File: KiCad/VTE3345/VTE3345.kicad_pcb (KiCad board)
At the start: 2 copper layers, 58.4 x 55.9 mm, 26 parts, among them J1 Program, J2 Keypad, J3 Display, J4 Power, Q1 IRF540N, Q2 BD138, SW1 Reset, SW2 Mode, SW3 Switch, U1 ESP-12F, U2 AMS1117-3.3

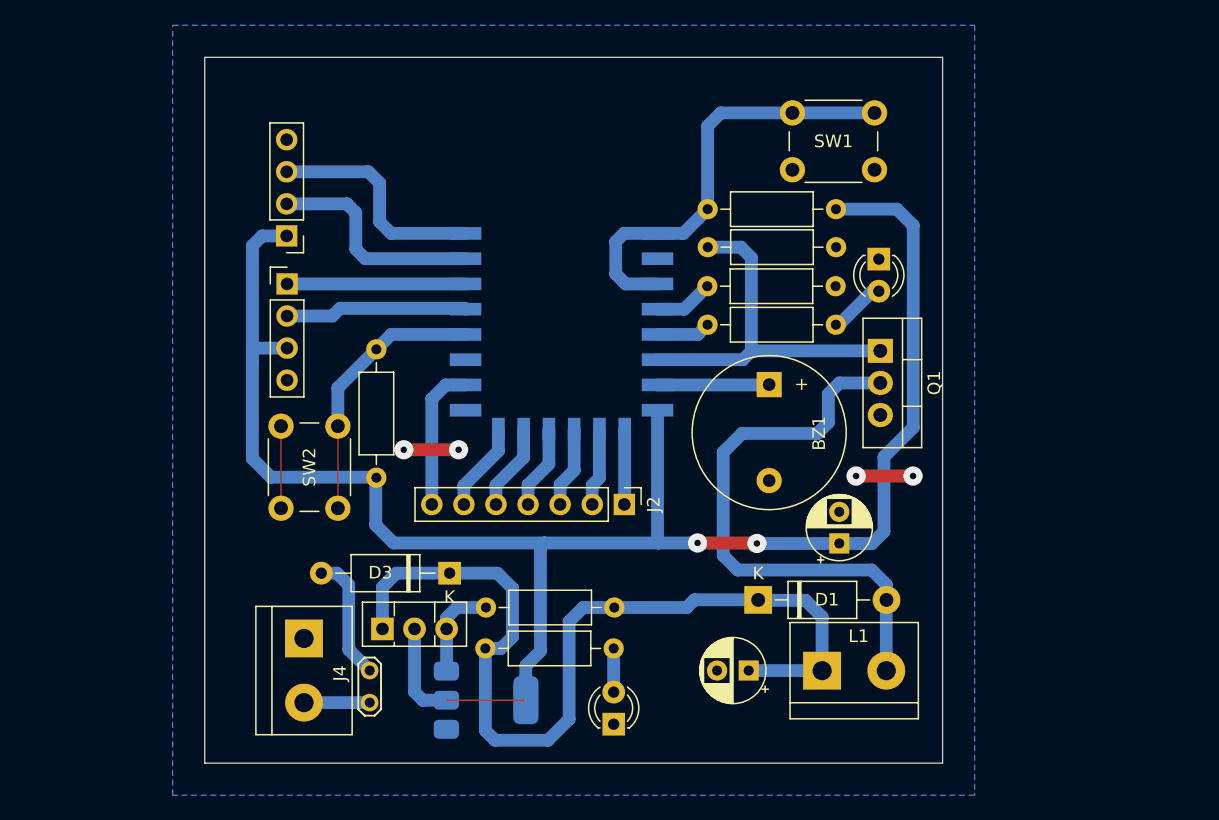
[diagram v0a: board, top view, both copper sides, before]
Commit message: Updates
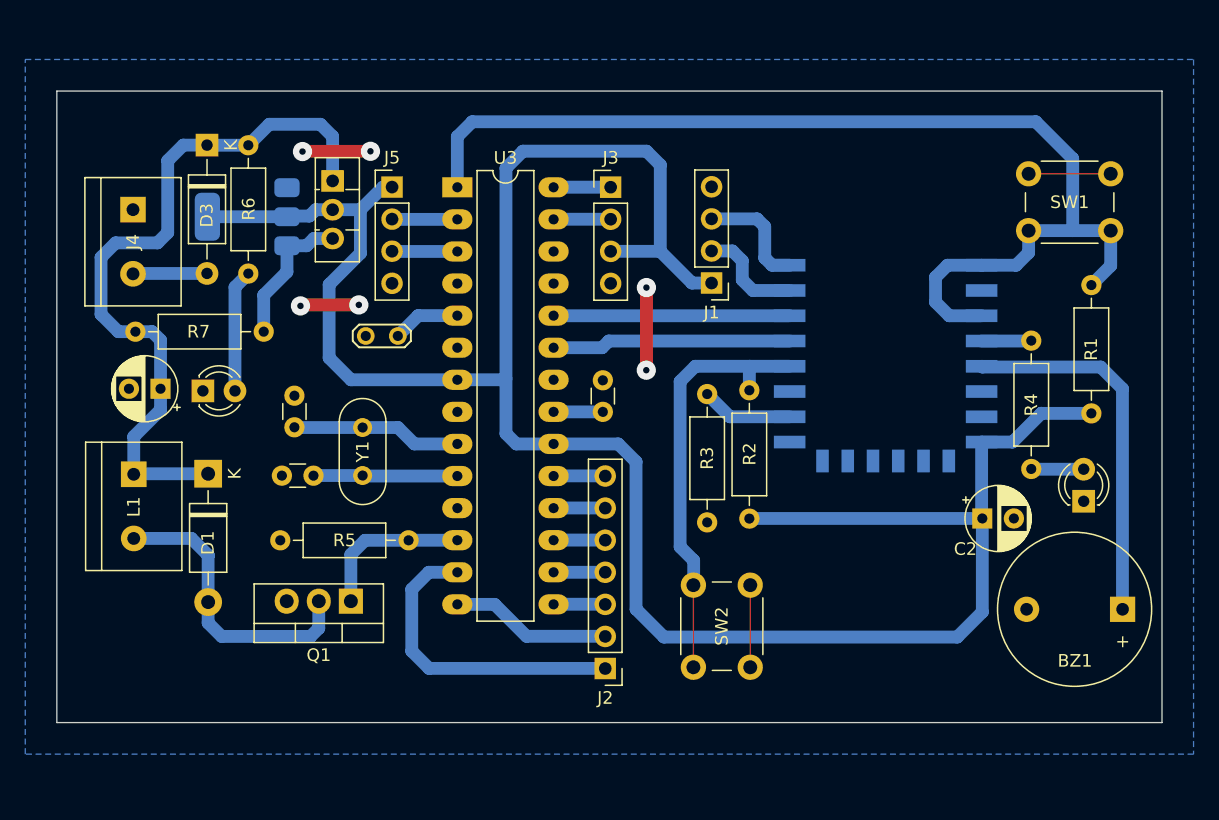
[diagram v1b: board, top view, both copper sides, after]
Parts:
- removed SW3: Switch, TestPoint:TestPoint_2Pads_Pitch2.54mm_Drill0.8mm
- added C3: 22pF, Capacitor_THT:C_Disc_D3.0mm_W1.6mm_P2.50mm, F.Cu at (126.7, 96.9)
- added C4: 22pF, Capacitor_THT:C_Disc_D3.0mm_W1.6mm_P2.50mm, F.Cu at (128.2, 100.7)
- added C5: 100nF, Capacitor_THT:C_Disc_D3.0mm_W1.6mm_P2.50mm, F.Cu at (151.2, 95.7)
- added J5: Program, Connector_PinHeader_2.54mm:PinHeader_1x04_P2.54mm_Vertical, F.Cu at (134.5, 77.9)
- added SW4: BTN, TestPoint:TestPoint_2Pads_Pitch2.54mm_Drill0.8mm, F.Cu at (134.9, 89.7)
- added U3: ATmega328P-P, Package_DIP:DIP-28_W7.62mm_LongPads, F.Cu at (139.6, 77.9)
- added Y1: 16MHz, Crystal:Crystal_HC52-U_Vertical, F.Cu at (132.1, 100.7)
- J1: value Program -> Program ESP
- moved L1 56.7 mm to (114.0, 100.6), turned to -90 degrees
- moved C1 51.6 mm to (116.1, 93.8)
- moved R5 49.8 mm to (125.6, 105.8), turned to 0 degrees
- moved Q1 46.4 mm to (131.2, 110.7), turned to 180 degrees
- moved D1 44.7 mm to (119.9, 100.6), turned to -90 degrees
- moved R6 44.0 mm to (123.1, 74.5), turned to -90 degrees
- moved R7 43.8 mm to (114.2, 89.3), turned to 0 degrees
- moved U2 42.7 mm to (123.0, 80.2), turned to 180 degrees
- moved D4 41.9 mm to (119.5, 94.0), turned to 0 degrees
- moved D3 39.0 mm to (119.8, 74.5), turned to -90 degrees
- moved J4 36.6 mm to (114.0, 79.7)
- moved Q2 35.7 mm to (129.8, 77.4), turned to -90 degrees
- moved SW2 34.0 mm to (158.3, 115.9), turned to 90 degrees
- moved J1 33.8 mm to (159.8, 85.5)
- moved BZ1 33.2 mm to (192.3, 111.3), turned to 180 degrees
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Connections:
- net /Rx renamed /RXD
- net /Tx renamed /TXD
- net Net-(SW1-B) renamed /reset
- J2 pad 1: /row1 -> /keypad_pin
- J2 pad 2: /row2 -> Net-(J2-Pin_2)
- J2 pad 3: /row3 -> Net-(J2-Pin_3)
- J2 pad 4: /row4 -> Net-(J2-Pin_4)
- J2 pad 5: /col1 -> Net-(J2-Pin_5)
- J2 pad 6: /col2 -> Net-(J2-Pin_6)
- J2 pad 7: /col3 -> Net-(J2-Pin_7)
- J4 pad 2: Net-(J4-Pin_2) -> Net-(D3-A)
- R3 pad 1: Net-(U1-GPIO16) -> Net-(U1-GPIO15)
- R4 pad 1: Net-(U1-GPIO14) -> Net-(U1-GPIO16)
- U1 pad 10: /row2 -> unconnected-(U1-MISO-Pad10)
- U1 pad 11: /row3 -> unconnected-(U1-GPIO9-Pad11)
- U1 pad 12: /row4 -> unconnected-(U1-GPIO10-Pad12)
- U1 pad 13: /col1 -> unconnected-(U1-MOSI-Pad13)
- U1 pad 14: /col2 -> unconnected-(U1-SCLK-Pad14)
- U1 pad 16: /col3 -> Net-(U1-GPIO15)
- U1 pad 19: /SDA -> /RxD
- U1 pad 20: /SCL -> /TxD
- U1 pad 5: Net-(U1-GPIO14) -> Net-(BZ1-+)
- U1 pad 6: Net-(Q1-G) -> unconnected-(U1-GPIO12-Pad6)
- U1 pad 7: Net-(BZ1-+) -> unconnected-(U1-GPIO13-Pad7)
- U1 pad 9: /row1 -> unconnected-(U1-CS0-Pad9)
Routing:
- net /reset: track 34.8 -> 87.6 mm
- net +3.3V: track 149.0 -> 187.2 mm, vias 4 -> 0
- net /keypad_pin: track 0.00 -> 25.0 mm
- net Net-(D1-A): track 44.9 -> 23.4 mm
- net Net-(BZ1-+): track 8.85 -> 29.4 mm
- net /RxD: track 0.00 -> 18.9 mm
- net /TxD: track 0.00 -> 18.7 mm
- net +12V: track 74.2 -> 57.5 mm
- net Net-(Q1-G): track 29.1 -> 12.6 mm
- net GND: track 15.3 -> 29.6 mm, vias 4 -> 6
- net Net-(U3-XTAL1/PB6): track 0.00 -> 13.4 mm
- net Net-(SW2-A): track 21.4 -> 34.2 mm
- net Net-(J2-Pin_2): track 0.00 -> 12.8 mm
- net /col3: track 11.5 -> 0.00 mm
- net Net-(U3-XTAL2/PB7): track 0.00 -> 11.4 mm
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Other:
- board size 58.4 x 55.9 mm -> 87.5 x 50 mm
